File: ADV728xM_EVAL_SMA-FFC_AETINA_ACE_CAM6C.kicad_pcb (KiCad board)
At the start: 2 copper layers, 86.5 x 33.6 mm, 16 parts, among them J1 142-0701-801, J2 142-0701-801, J3 142-0701-801, J4 142-0701-801, J5 Conn_01x04_Male, J6 Conn_01x04_Male, J7 Conn_01x02_Male, J8 Conn_01x02_Male, J9 3-1734742-6, U1 NLSX5014DTR2G

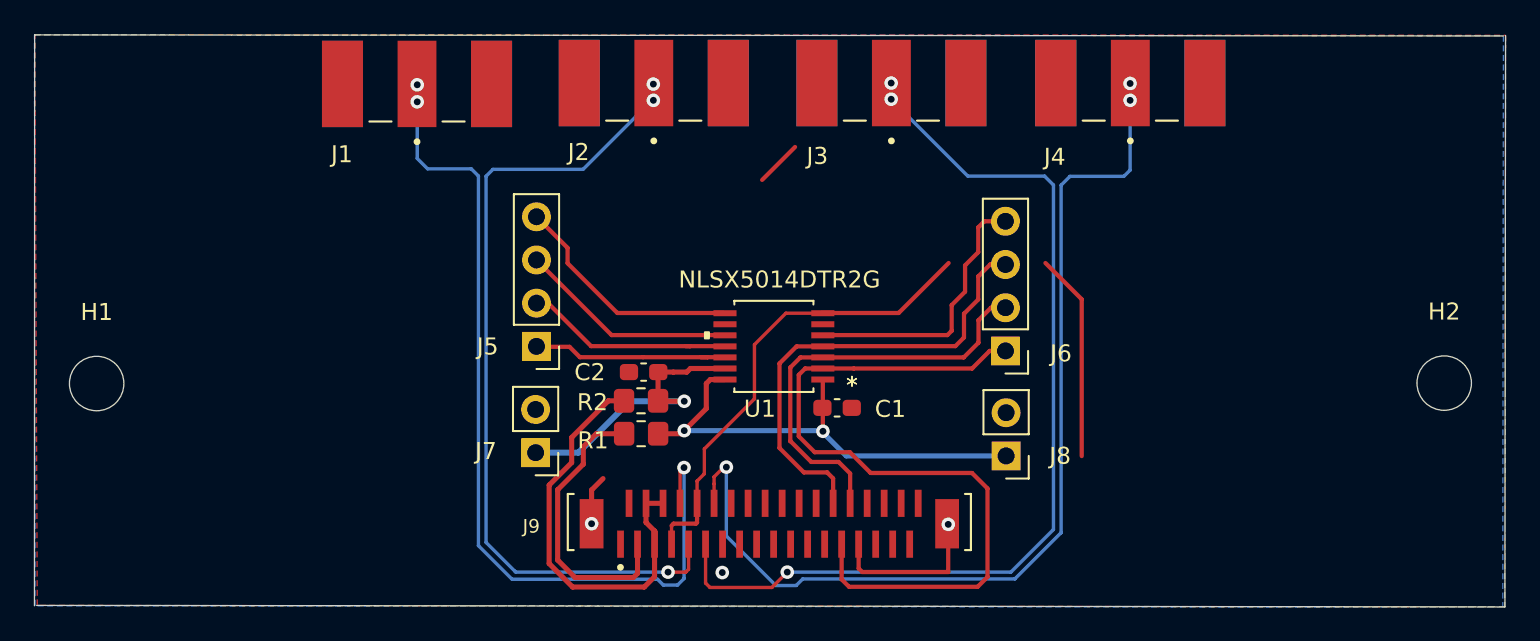
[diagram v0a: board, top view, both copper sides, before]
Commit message: Add production release V1A with board outline
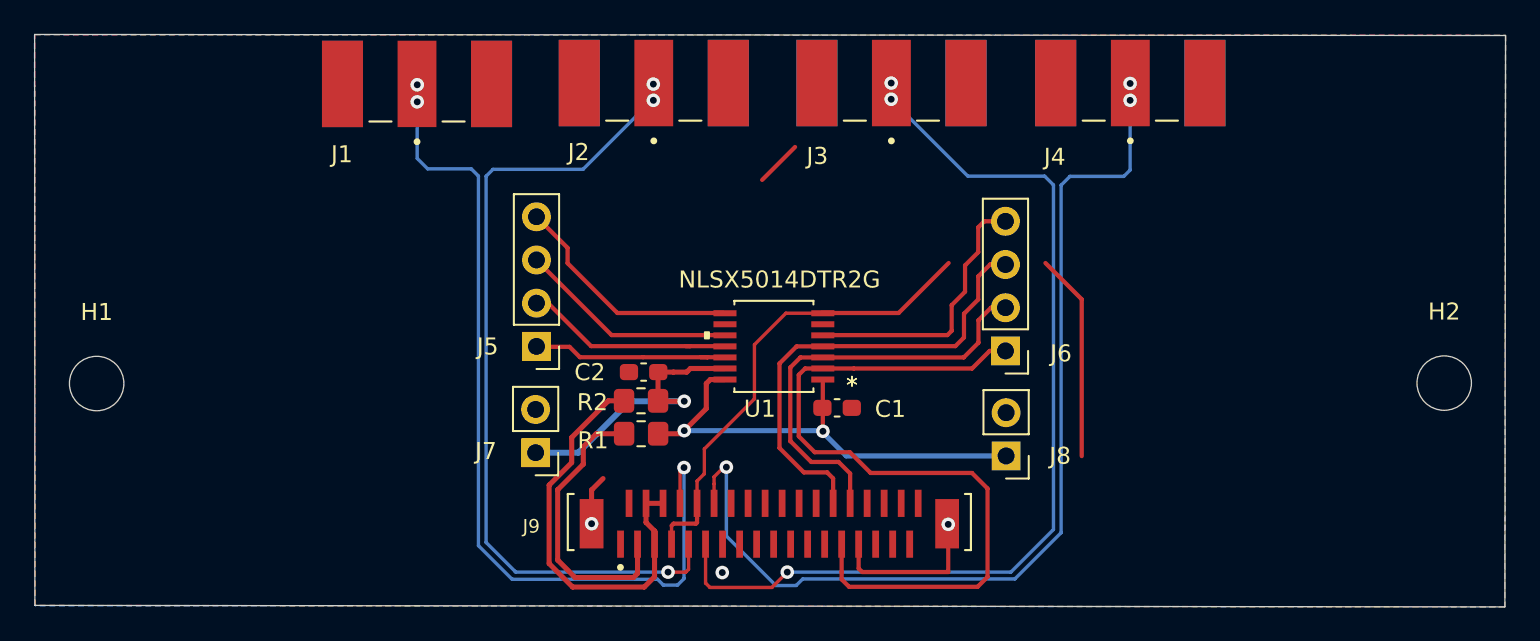
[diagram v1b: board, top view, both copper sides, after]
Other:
- board size 86.5 x 33.6 mm -> 86.5 x 33.7 mm
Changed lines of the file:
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@@
     )
   )
-  (gr_line (start 115.57 109.7534) (end 115.5827 76.1873) (layer Edge.Cuts) (width 0.05))
-  (gr_line (start 202.0189 109.8169) (end 115.697 109.728) (layer Edge.Cuts) (width 0.05))
+  (gr_line (start 115.5954 109.728) (end 115.5827 76.1619) (layer Edge.Cuts) (width 0.05))
+  (gr_line (start 202.0189 109.8169) (end 115.5954 109.728) (layer Edge.Cuts) (width 0.05))
   (gr_line (start 202.057 76.2254) (end 202.0189 109.8169) (layer Edge.Cuts) (width 0.05))
-  (gr_line (start 115.5827 76.1873) (end 201.93 76.2508) (layer Edge.Cuts) (width 0.05))
+  (gr_line (start 115.5827 76.1619) (end 202.057 76.2254) (layer Edge.Cuts) (width 0.05))
   (segment (start 152.2465 97.7403) (end 152.2349 97.7519) (width 0.35) (layer F.Cu) (net 1))
   (segment (start 154.1318 95.8007) (end 154.1272 95.7961) (width 0.25) (layer F.Cu) (net 1))
@@
     (polygon
       (pts
-        (xy 202.057 76.2127) (xy 202.0189 109.8169) (xy 115.7351 109.728) (xy 115.5954 76.1746)
+        (xy 202.057 76.2127) (xy 202.0189 109.8169) (xy 115.6081 109.728) (xy 115.5954 76.1746)
       )
     )
@@
     (polygon
       (pts
-        (xy 201.93 76.238033) (xy 201.8919 109.842233) (xy 115.6081 109.753333) (xy 115.57 76.187233)
+        (xy 202.057 76.2127) (xy 202.0189 109.8169) (xy 115.6081 109.753333) (xy 115.57 76.187233)
       )
     )
